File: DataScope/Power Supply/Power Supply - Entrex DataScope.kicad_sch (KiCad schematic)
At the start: 128 parts, among them J2 Power Port, Q1 MPS3638, Q10 PN3569, Q11 PS3638, Q12 2N4918, Q13 2N3055, Q14 PN3569, Q15 PS3638, Q16 PN3569, Q17 PN3569, Q18 PS3638, Q19 JE520, Q2 PN3569, Q20 PN3569, Q3 PN3569, Q4 PS3638, Q5 2N4918, Q6 2N3055, Q7 PN3569, Q8 PS3638, Q9 PN3569

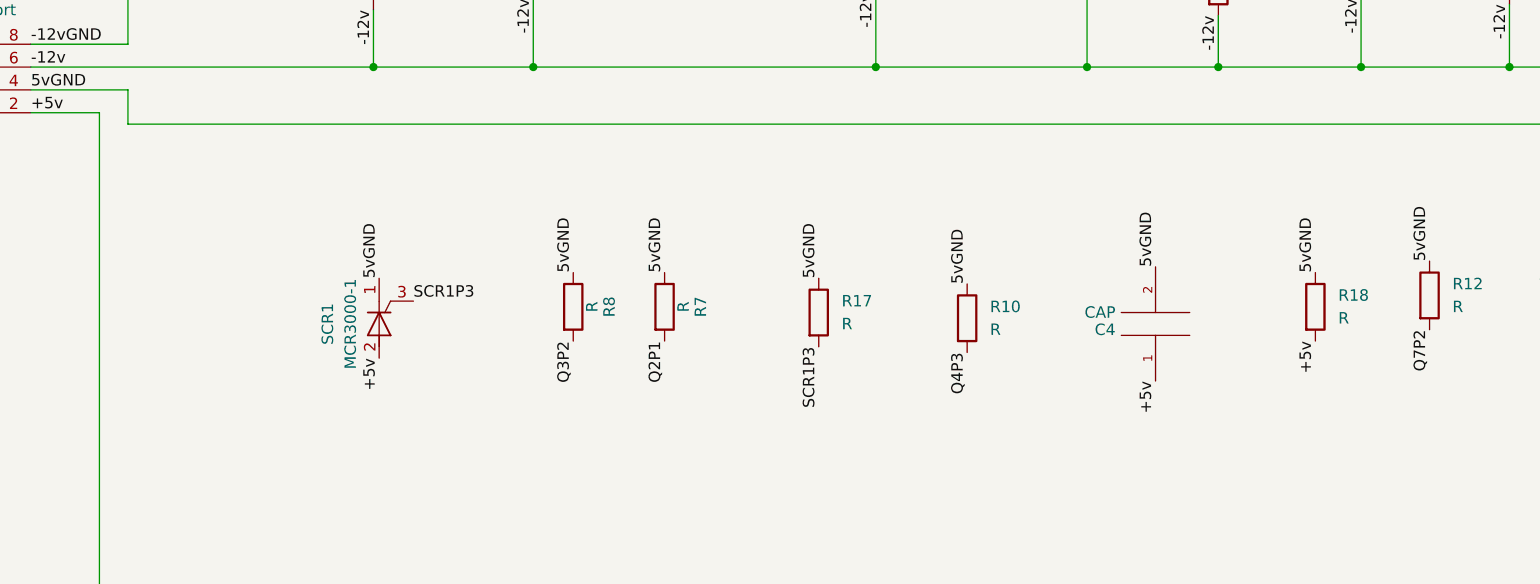
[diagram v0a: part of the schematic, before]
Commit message: build
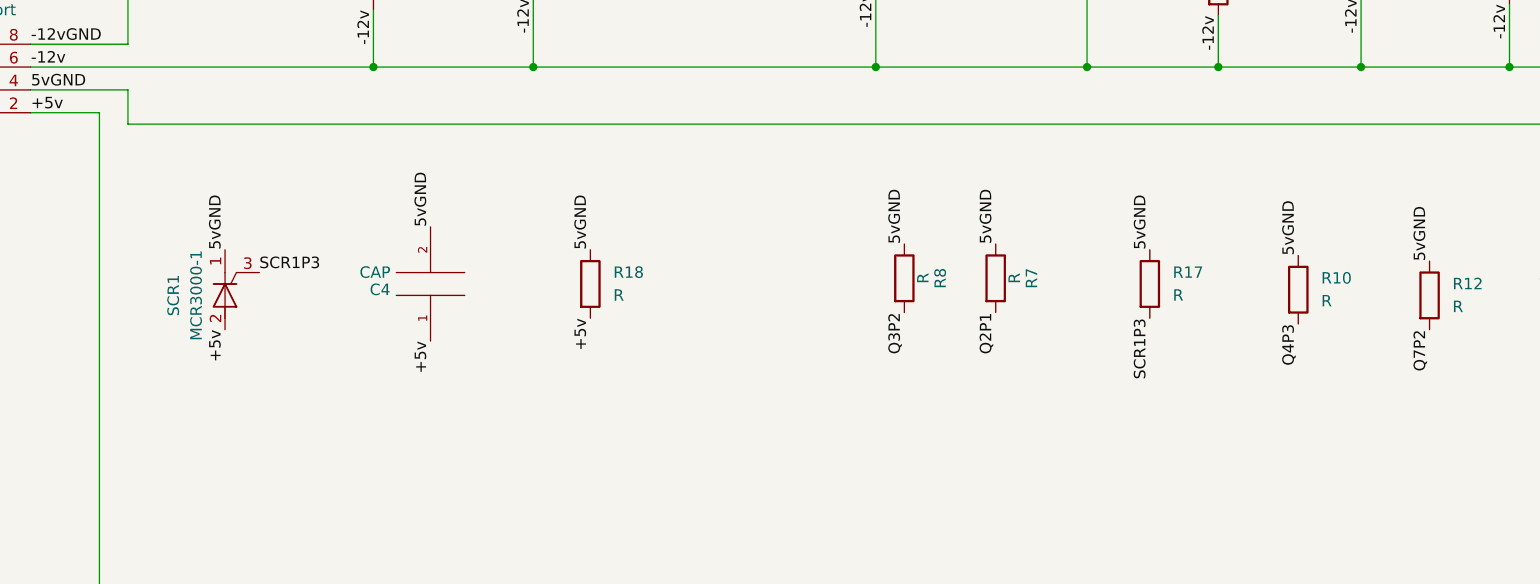
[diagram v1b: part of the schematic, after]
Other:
- moved on the sheet: C4, R10, R17, R18, R7, R8, SCR1

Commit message: build
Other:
- moved on the sheet: CR7, Q3, Q7, R13, R15, R8

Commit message: Build
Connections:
- net Q13P2: now also R32.1
- net Q14P2: now also R30.2
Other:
- moved on the sheet: C1, C10, C11, C12, C3, C4, C5, C6, C7, C8, C9, CR1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
